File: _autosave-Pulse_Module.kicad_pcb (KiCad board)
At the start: 2 copper layers, 20.1 x 17.2 mm, 61 parts, among them CON1 AVR-ISP-10, CON2 AVR-JTAG-10, IC1 ATMEGA1280-A, P1 CONN_02X20, P2 USB_OTG, SW1 SW_PUSH, U1 74HCT541_PWR, U2 PL2303, U5 CONN3, U6 WS2812, U7 WS2812, U8 WS2812, U9 CONN3, X1 CRYSTAL, Y1 CRYSTAL

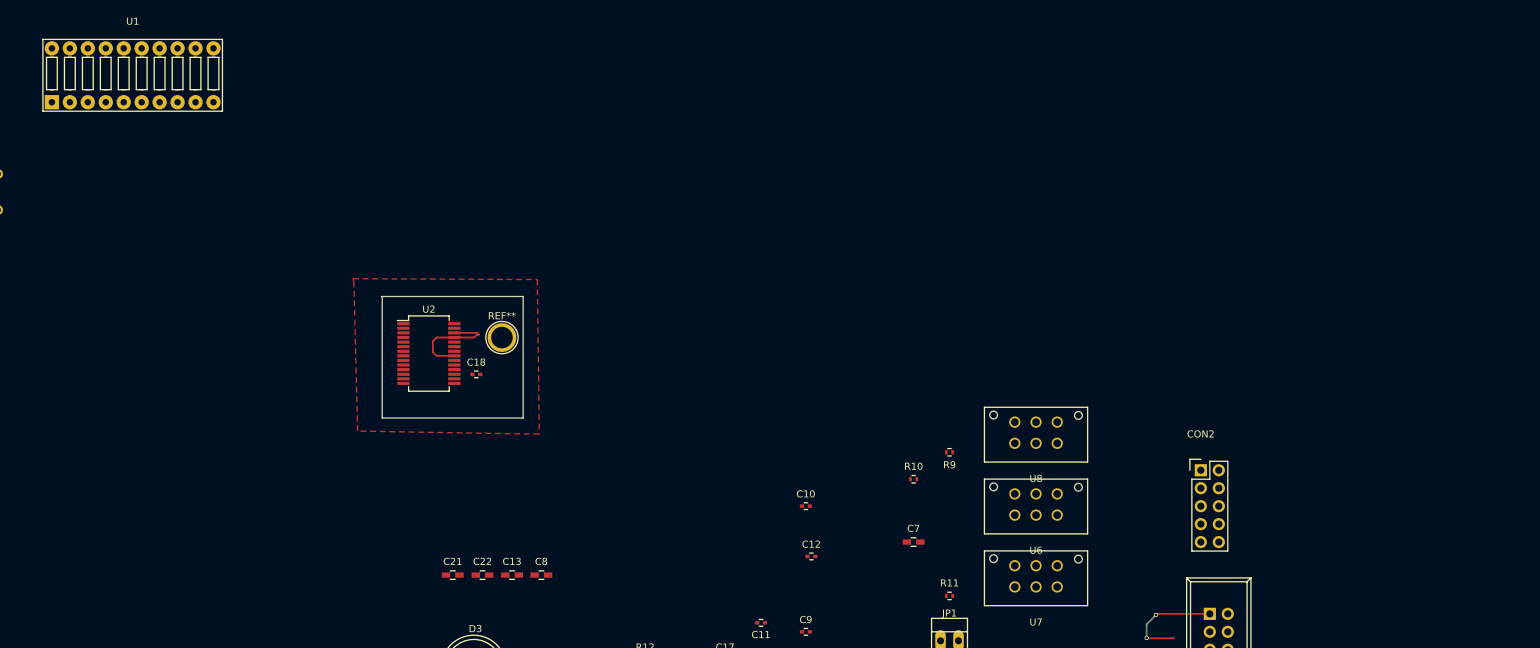
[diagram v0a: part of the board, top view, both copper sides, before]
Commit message: Небольшие изменения
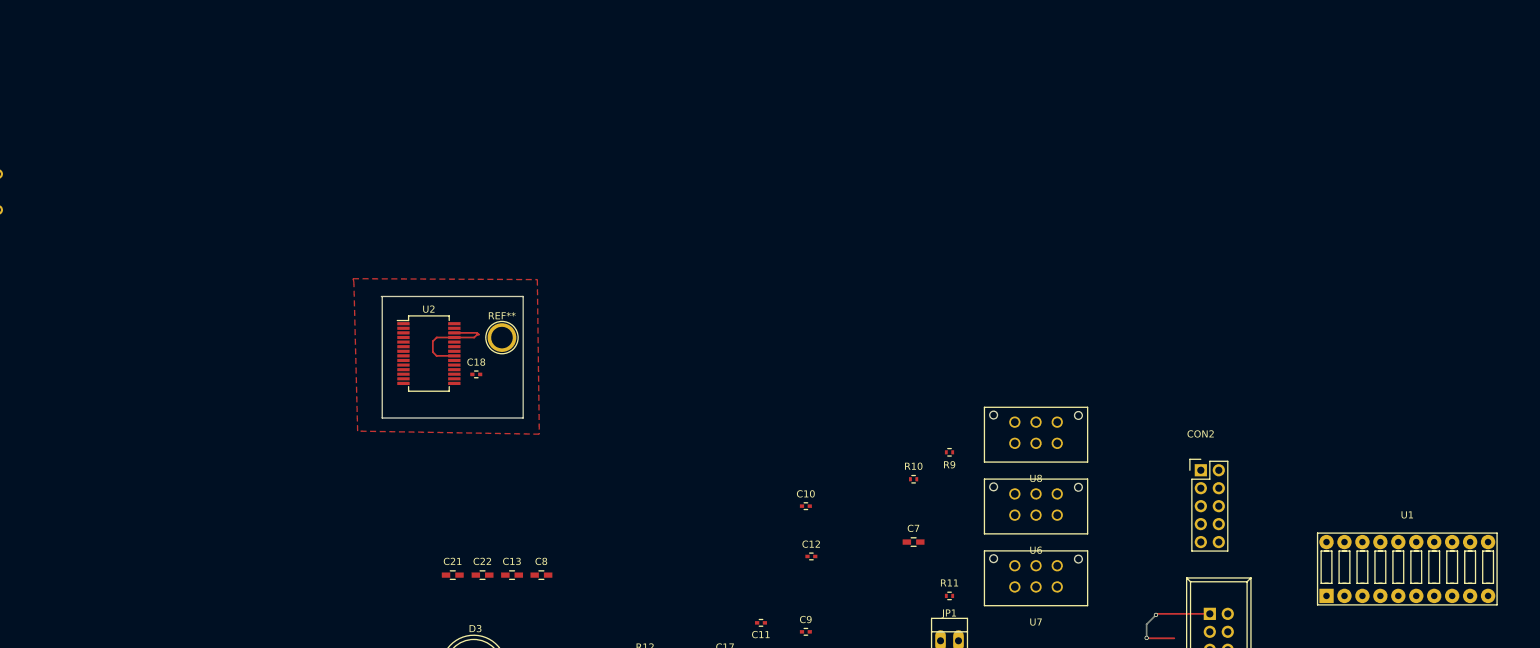
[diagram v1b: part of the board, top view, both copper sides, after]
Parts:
- moved U1 193.4 mm to (215.9, 73.7)
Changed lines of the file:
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@@
   )
   (module Display:HDSP-48xx (layer F.Cu)
-    (at 35.56 3.81)
+    (at 215.9 73.66)
     (descr "Barre 10 points")
     (tags BARGRAPH)
